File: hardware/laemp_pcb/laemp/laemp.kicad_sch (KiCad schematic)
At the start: 15 parts, among them J1 Conn_02x04_Counter_Clockwise, J2 Conn_01x02_Pin, U1 TPS61165DBV, U2 TPS61165DBV, U3 TPS61165DBV, U4 TPS61165DBV, U5 TPS54202DDC

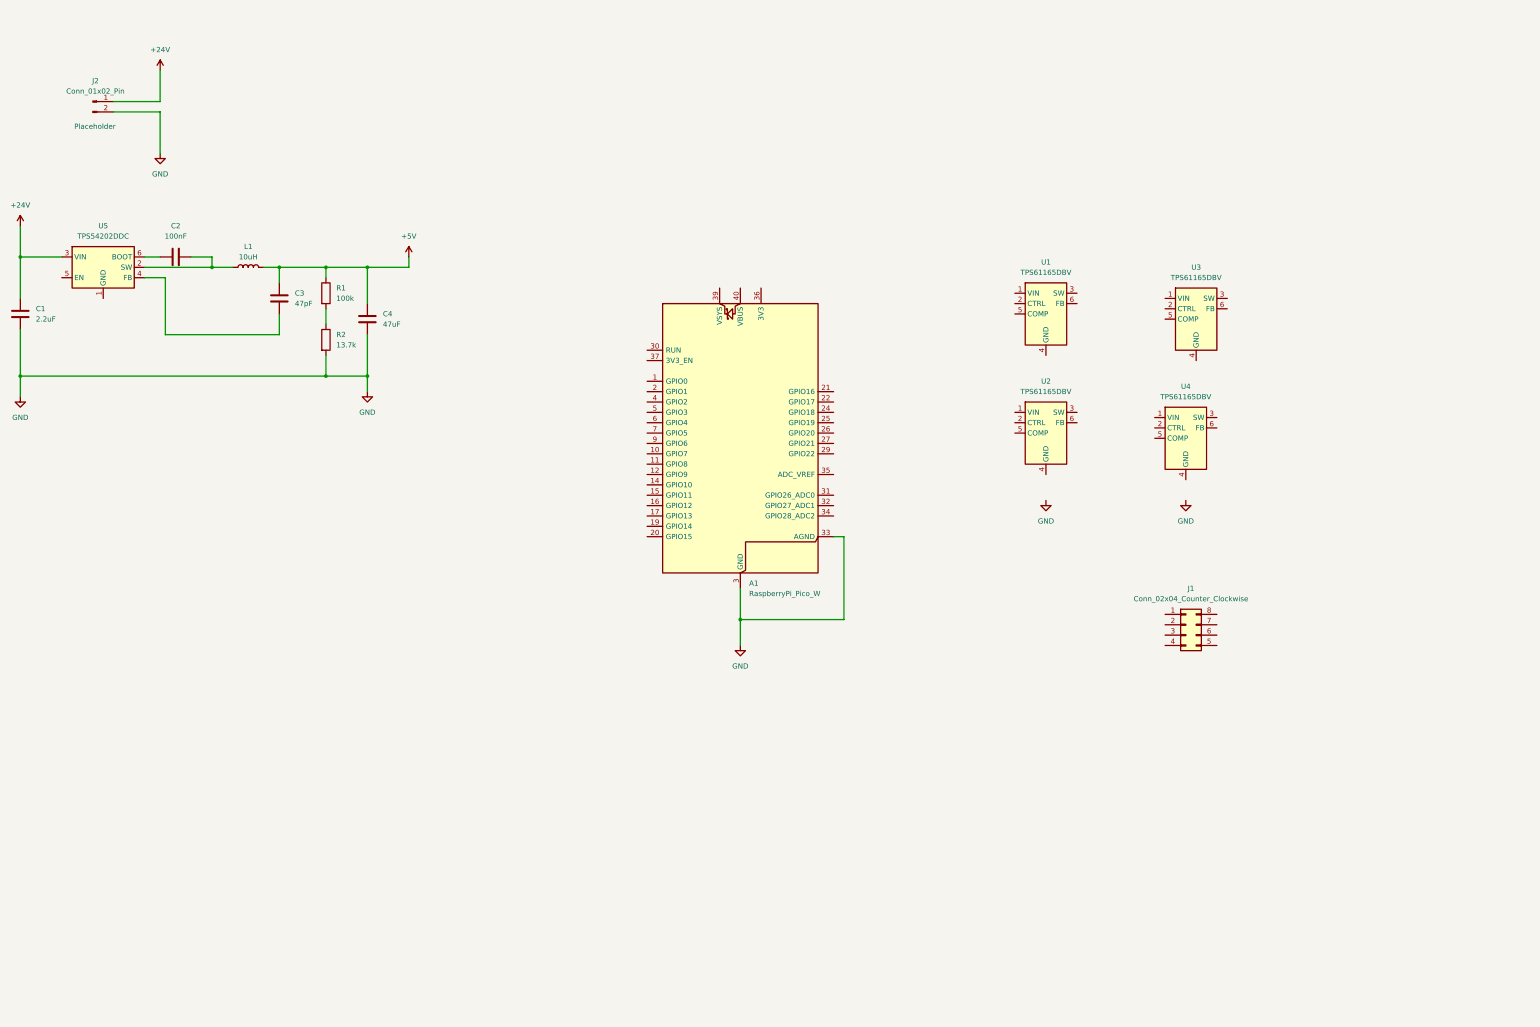
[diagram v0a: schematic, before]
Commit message: driver layout
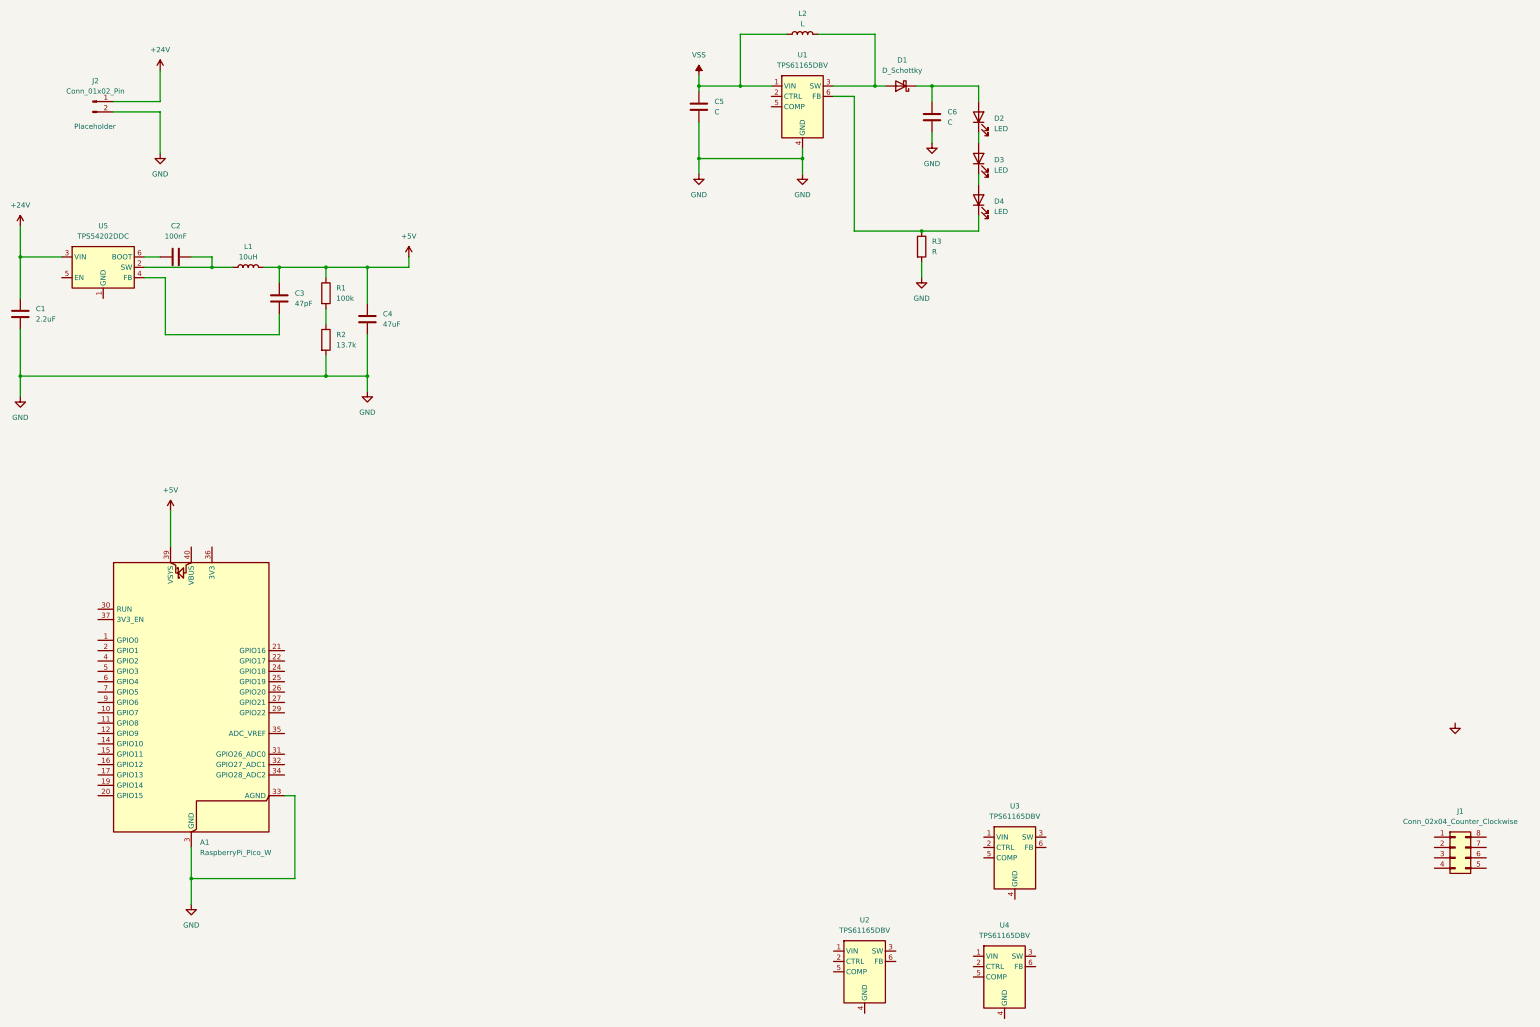
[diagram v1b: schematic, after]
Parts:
- added C5, C6: C, symbol Device:C
- added D1: D_Schottky, symbol Device:D_Schottky
- added D2, D3, D4: LED, symbol Device:LED
- added L2: L, symbol Device:L
- added R3: R, symbol Device:R
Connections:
- net +5V: now also A1.39 (VSYS)
- net GND: now also U1.4 (GND), C5.2, C6.2, R3.2
- net VSS: now reaches U1.1 (VIN)
- net VSS: now also C5.1, L2.1
- net at U1.3 (SW): now also D1.2 (A), L2.2
- net at U1.6 (FB): now also D4.1 (K), R3.1
- new net: D3.1 (K), D4.2 (A)
- new net: C6.1, D1.1 (K), D2.2 (A)
- new net: D2.1 (K), D3.2 (A)
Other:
- moved on the sheet: A1, J1, U1, U2, U3, U4
